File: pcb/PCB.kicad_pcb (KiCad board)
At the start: 4 copper layers, 86.4 x 27.9 mm, 57 parts, among them J1 Micro_SD_Card, J2 JST B04b-XASK, J3 JST B04B-XASK, J4 0.1 INCH HEADER, J5 TC2030, J6 0.1 INCH HEADER, U1 SN65HVD230, U2 XBPRO-900, U4 STM32F412RETx, U5 SN65HVD230, Y2 8MHz

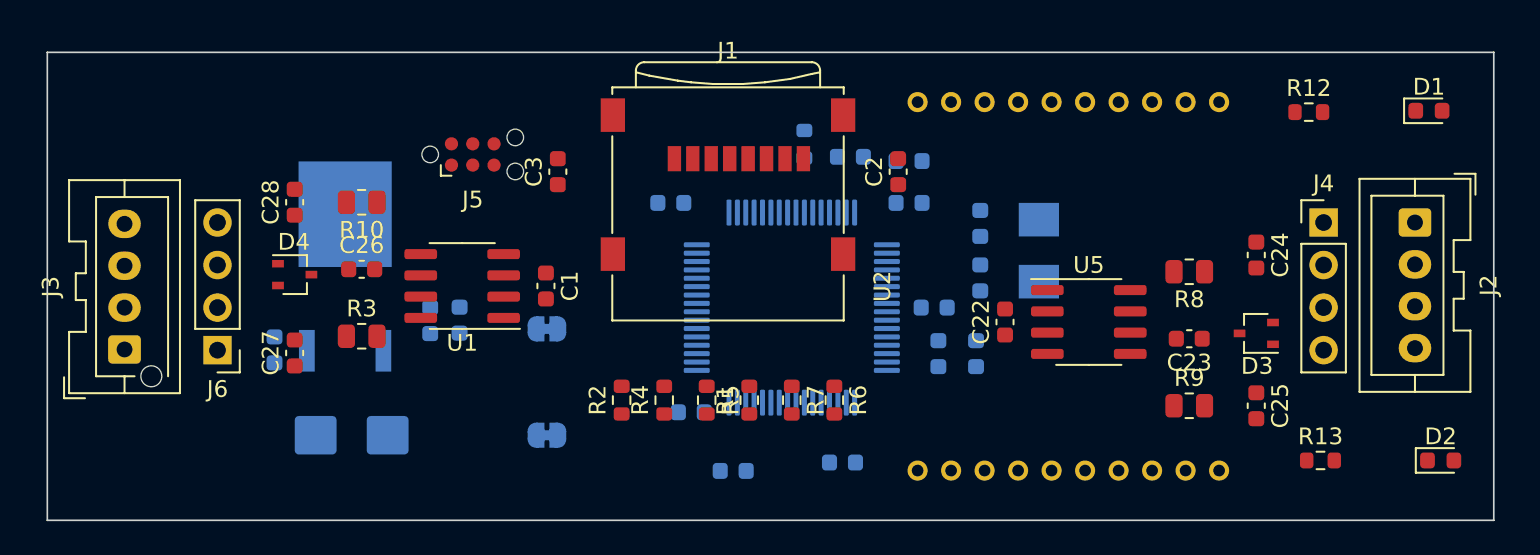
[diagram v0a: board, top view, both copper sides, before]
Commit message: Finished Telemetry PCB
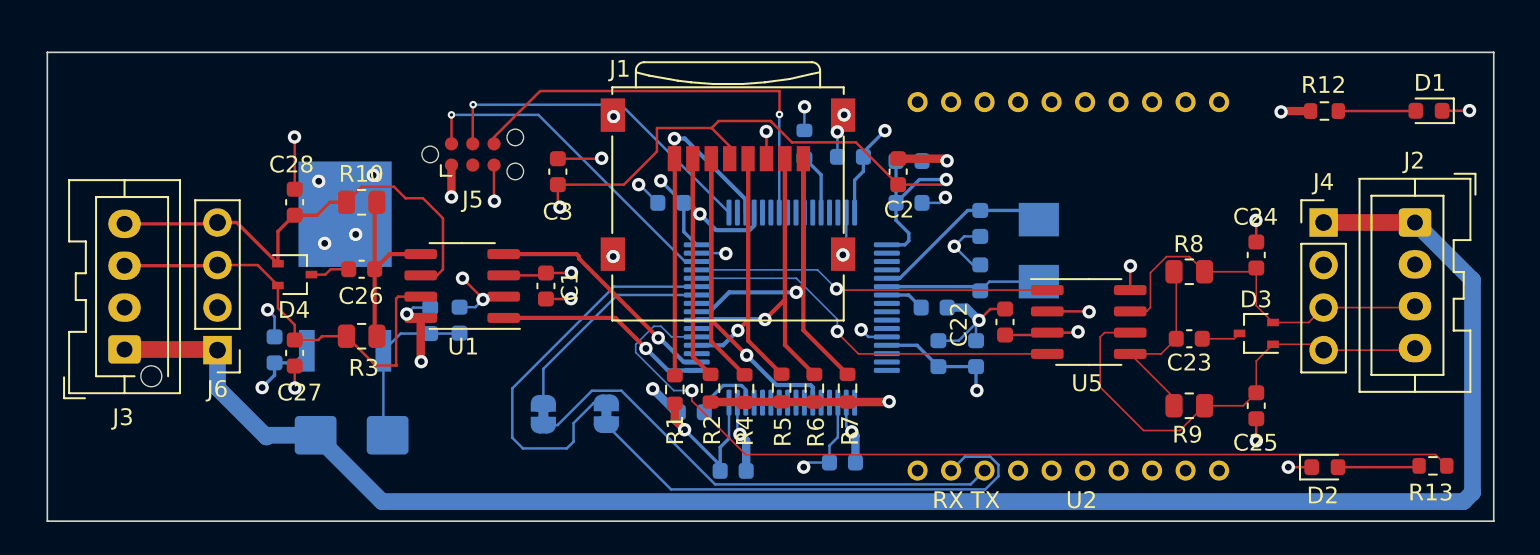
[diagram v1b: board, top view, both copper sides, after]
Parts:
- added G***: LOGO, toucan:toucan, B.Cu at (182.0, 70.4)
- moved D2 6.93 mm to (190.1, 78.9)
- moved R13 6.72 mm to (196.5, 78.8)
- moved R2 5.36 mm to (153.4, 74.2)
- moved JP2 5.10 mm to (143.4, 75.7), turned to 90 degrees
- moved R4 4.85 mm to (155.4, 74.2)
- moved R5 4.53 mm to (157.6, 74.1)
- moved R1 4.49 mm to (151.3, 74.2)
- moved JP1 3.77 mm to (147.2, 75.7), turned to 90 degrees
- moved R7 3.40 mm to (161.6, 74.2)
- moved R6 1.39 mm to (159.6, 74.2)
- moved R12 0.94 mm to (190.0, 57.6), turned to 180 degrees
- turned D1 to 180 degrees
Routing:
- net +12V: track 0.00 -> 108.9 mm
- net +3V3: track 0.00 -> 100.6 mm, vias 0 -> 13
- net GND: track 0.00 -> 71.7 mm, vias 0 -> 37
- net MICROLED: track 0.00 -> 56.4 mm, vias 0 -> 1
- net SD-CMD: track 0.00 -> 32.0 mm, vias 0 -> 1
- net Net-(JP2-A): track 0.00 -> 29.9 mm
- net Net-(JP1-A): track 0.00 -> 29.4 mm
- net SD-DAT1: track 0.00 -> 28.5 mm, vias 0 -> 1
- net CAN2-: track 0.00 -> 28.4 mm
- net CAN1-: track 0.00 -> 28.2 mm
- net SD-DAT0: track 0.00 -> 27.8 mm, vias 0 -> 1
- net SD-CLK: track 0.00 -> 27.0 mm, vias 0 -> 1
- net SWO: track 0.00 -> 25.8 mm, vias 0 -> 1
- net CAN2+: track 0.00 -> 25.8 mm
- net UART-RX: track 0.00 -> 24.1 mm
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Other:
- board size 86.4 x 27.9 mm -> 86.4 x 28 mm
- board text added: "12V"
- board text added: "CAN1+"
- board text added: "CAN1-"
- board text added: "CAN2+"
- board text added: "CAN2-"
- board text added: "GND"
- board text added: "Leo Lake Bronco Racing Telemetry Board Rev 2 JAN 2024"
- board text added: "RX"
- board text added: "TX"
